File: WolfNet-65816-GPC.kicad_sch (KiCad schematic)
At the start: 37 parts, among them J1 Conn_01x01, J2 Conn_01x01, J3 Conn_01x01, J4 Conn_01x01, J5 USB_B, J6 ATX-24, SW1 SW_SPST, SW2 SW_Push, U1 WD65C816S, U10 LM7905_TO220, U11 SC28L91, U12 DS1813, U2 MCP2200-I-SO, U3 74HCT573, U4 74HCT245, U5 AS6C1608, U6 XCR3064XL-VQ100, U7 SST39SF040, U8 SST39SF040, U9 XCR3064XL-VQ100, X1 ACO-12MHz, X2 ACO-3.6864MHz

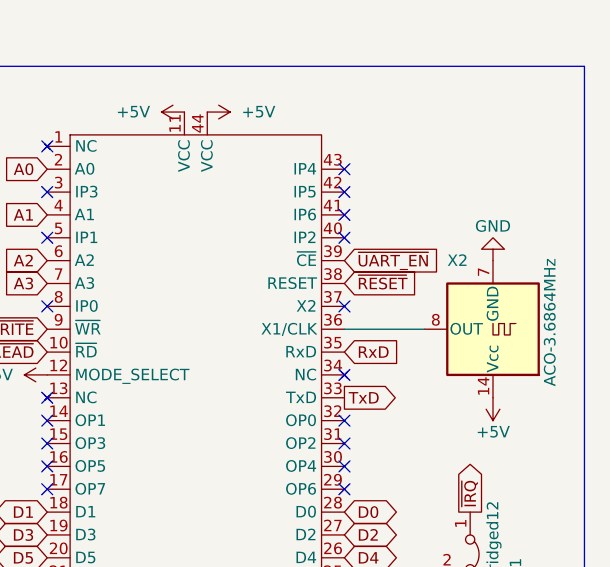
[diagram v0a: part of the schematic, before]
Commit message: Update WolfNet-65816-GPC.kicad_sch
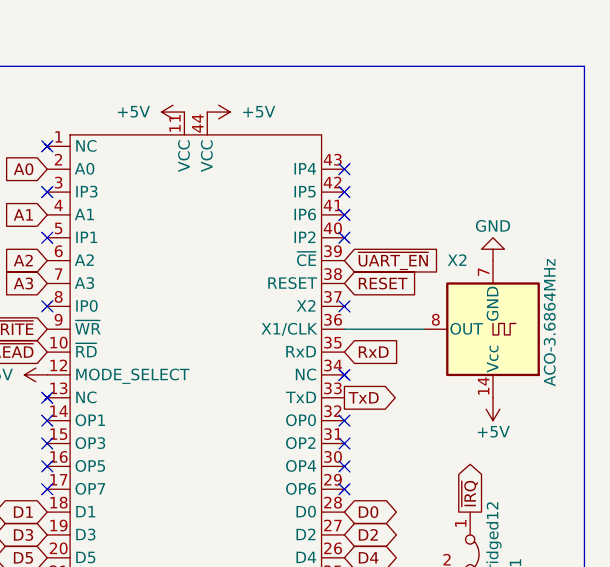
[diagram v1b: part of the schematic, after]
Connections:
- net ~{RESET}: no longer U11.38 (RESET)
- new net RESET: U11.38 (RESET)
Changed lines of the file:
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@@
     )
   )
-  (global_label "~{RESET}" (shape input) (at 378.46 39.37 0) (fields_autoplaced)
+  (global_label "RESET" (shape input) (at 378.46 39.37 0) (fields_autoplaced)
     (effects (font (size 1.27 1.27)) (justify left))
     (property "Intersheet References" "${INTERSHEET_REFS}" (id 0) (at 386.6183 39.2906 0)
